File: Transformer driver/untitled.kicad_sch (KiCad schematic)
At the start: 0 parts

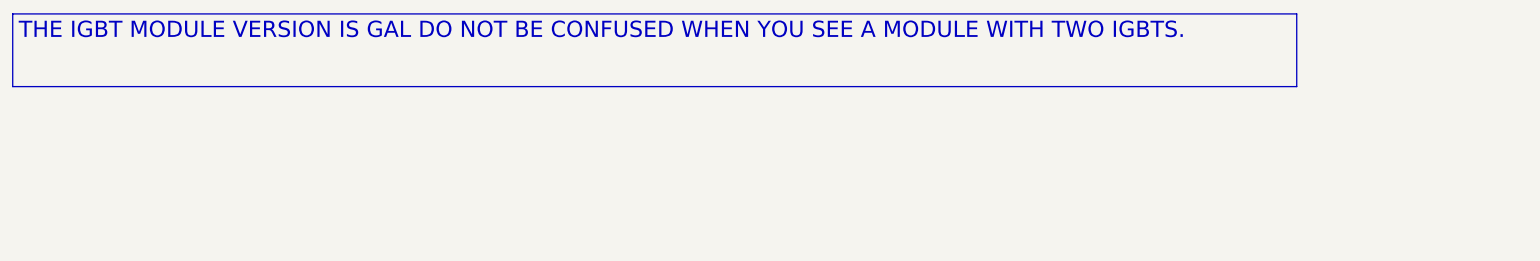
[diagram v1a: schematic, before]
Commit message: commits
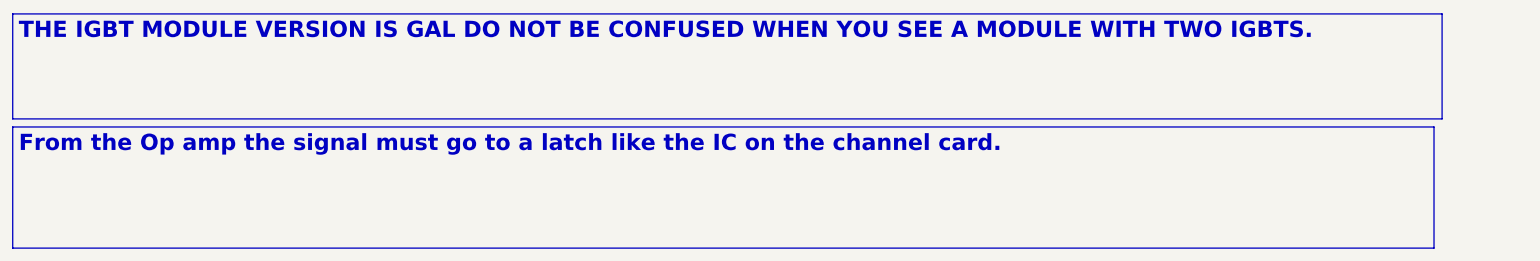
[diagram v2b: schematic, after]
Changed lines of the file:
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@@
 		(exclude_from_sim no)
 		(at 17.78 19.05 0)
-		(size 201.93 11.43)
+		(size 224.79 16.51)
 		(margins 0.9525 0.9525 0.9525 0.9525)
 		(stroke
@@
 			(font
 				(size 2.54 2.54)
+				(thickness 0.508)
+				(bold yes)
 			)
 			(justify left top)
+		)
+	)
+	(text_box "From the Op amp the signal must go to a latch like the IC on the channel card."
+		(exclude_from_sim no)
+		(at 17.78 36.83 0)
+		(size 223.52 19.05)
+		(margins 0.9525 0.9525 0.9525 0.9525)
+		(stroke
+			(width 0)
+			(type solid)
+		)
+		(fill
+			(type none)
+		)
+		(effects
+			(font
+				(size 2.54 2.54)
+				(thickness 0.508)
+				(bold yes)
+			)
+			(justify left top)
